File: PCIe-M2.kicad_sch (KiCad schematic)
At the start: 24 parts, among them J4 Bus_M.2_Socket_M, M1 M.2 Screw, M2 M.2 Solder Nut, M3 M.2 Solder Nut, M4 M.2 Solder Nut, M5 M.2 Solder Nut, U7 ASEK-32.768KHZ-L-R-T, U8 AP3441SHE-7B

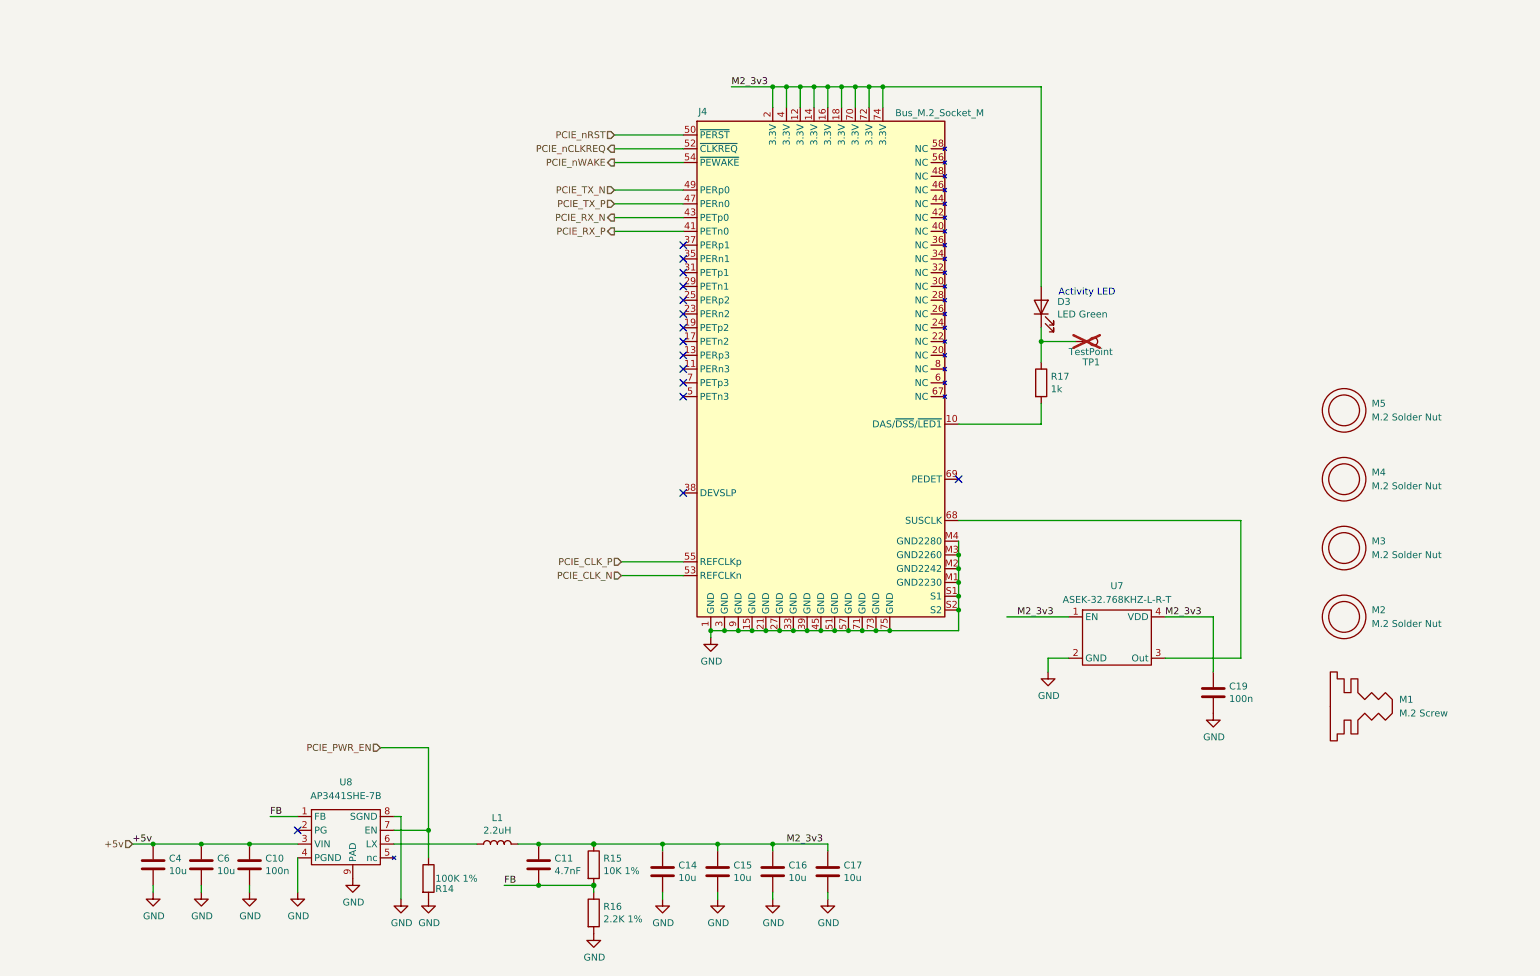
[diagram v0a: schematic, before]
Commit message: add modifications so far
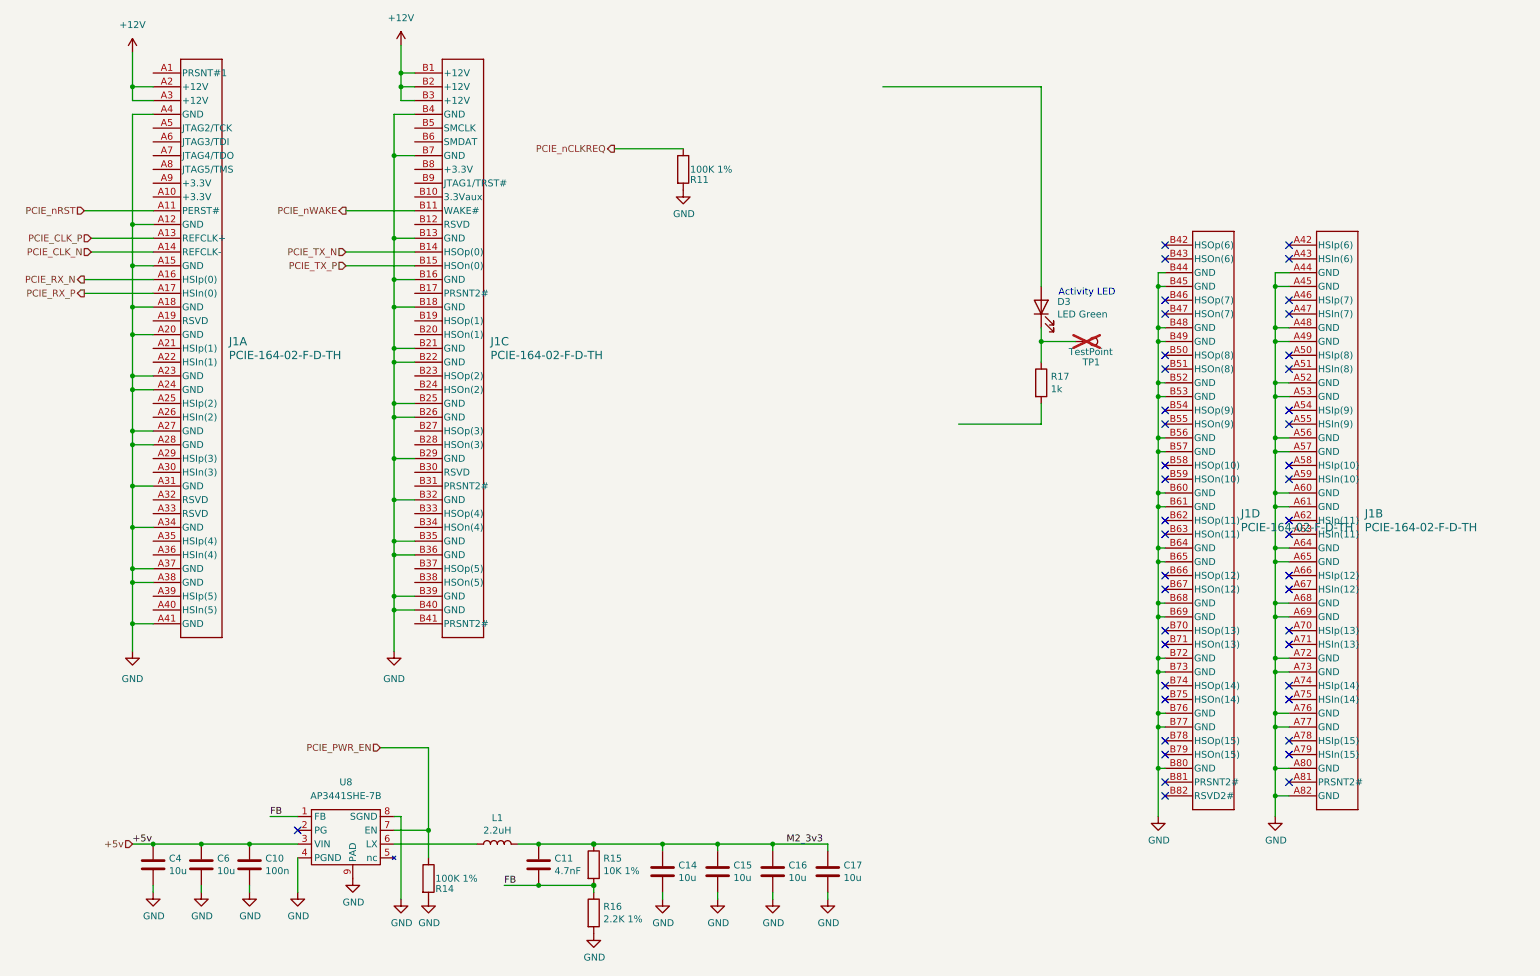
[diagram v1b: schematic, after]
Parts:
- removed C19: 100n, Capacitor_SMD:C_0402_1005Metric, symbol Device:C
- removed J4: Bus_M.2_Socket_M, CM5IO:M.2 M Key socket, symbol CM5IO:Bus_M.2_Socket_M
- removed M1: M.2 Screw, symbol CM5IO:M.2_Screw
- removed M2, M3, M4, M5: M.2 Solder Nut, symbol CM5IO:SolderNut
- removed U7: ASEK-32.768KHZ-L-R-T, Crystal:Crystal_SMD_3225-4Pin_3.2x2.5mm, symbol CM5IO:ASEK-32.768KHZ-L-R-T
- added J1: PCIE-164-02-F-D-TH, CONN_PCIE-164-02-x-D-TH_SAI, symbol CM5IO:PCIE-164-02-F-D-TH
- added R11: 100K 1%, Resistor_SMD:R_0402_1005Metric, symbol Device:R
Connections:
- net GND: now also J1.A12 (GND), J1.A15 (GND), J1.A18 (GND), J1.A20 (GND), J1.A23 (GND), J1.A24 (GND), J1.A27 (GND), J1.A28 (GND), J1.A31 (GND), J1.A34 (GND), J1.A37 (GND), J1.A38 (GND), J1.A4 (GND), J1.A41 (GND), J1.A44 (GND), J1.A45 (GND), J1.A48 (GND), J1.A49 (GND), J1.A52 (GND), J1.A53 (GND), J1.A56 (GND), J1.A57 (GND), J1.A60 (GND), J1.A61 (GND), J1.A64 (GND), J1.A65 (GND), J1.A68 (GND), J1.A69 (GND), J1.A72 (GND), J1.A73 (GND), J1.A76 (GND), J1.A77 (GND), J1.A80 (GND), J1.A82 (GND), J1.B13 (GND), J1.B16 (GND), J1.B18 (GND), J1.B21 (GND), J1.B22 (GND), J1.B25 (GND), J1.B26 (GND), J1.B29 (GND), J1.B32 (GND), J1.B35 (GND), J1.B36 (GND), J1.B39 (GND), J1.B4 (GND), J1.B40 (GND), J1.B44 (GND), J1.B45 (GND), J1.B48 (GND), J1.B49 (GND), J1.B52 (GND), J1.B53 (GND), J1.B56 (GND), J1.B57 (GND), J1.B60 (GND), J1.B61 (GND), J1.B64 (GND), J1.B65 (GND), J1.B68 (GND), J1.B69 (GND), J1.B7 (GND), J1.B72 (GND), J1.B73 (GND), J1.B76 (GND), J1.B77 (GND), J1.B80 (GND), R11.2
- net M2_3v3: no longer D3.2 (A)
- net PCIE_CLK_N: now also J1.A14 (REFCLK-)
- net PCIE_CLK_P: now also J1.A13 (REFCLK+)
- net PCIE_RX_N: now also J1.A16 (HSIp(0))
- net PCIE_RX_P: now also J1.A17 (HSIn(0))
- net PCIE_TX_N: now also J1.B14 (HSOp(0))
- net PCIE_TX_P: now also J1.B15 (HSOn(0))
- net PCIE_nCLKREQ: now also R11.1
- net PCIE_nRST: now also J1.A11 (PERST#)
- net PCIE_nWAKE: now also J1.B11 (WAKE#)
- new net +12V: J1.A2 (+12V), J1.A3 (+12V), J1.B1 (+12V), J1.B2 (+12V), J1.B3 (+12V)
- no-connect marks 15 -> 44
